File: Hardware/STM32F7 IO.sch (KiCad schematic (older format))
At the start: 19 parts, among them U16 STM32F765ZGT6

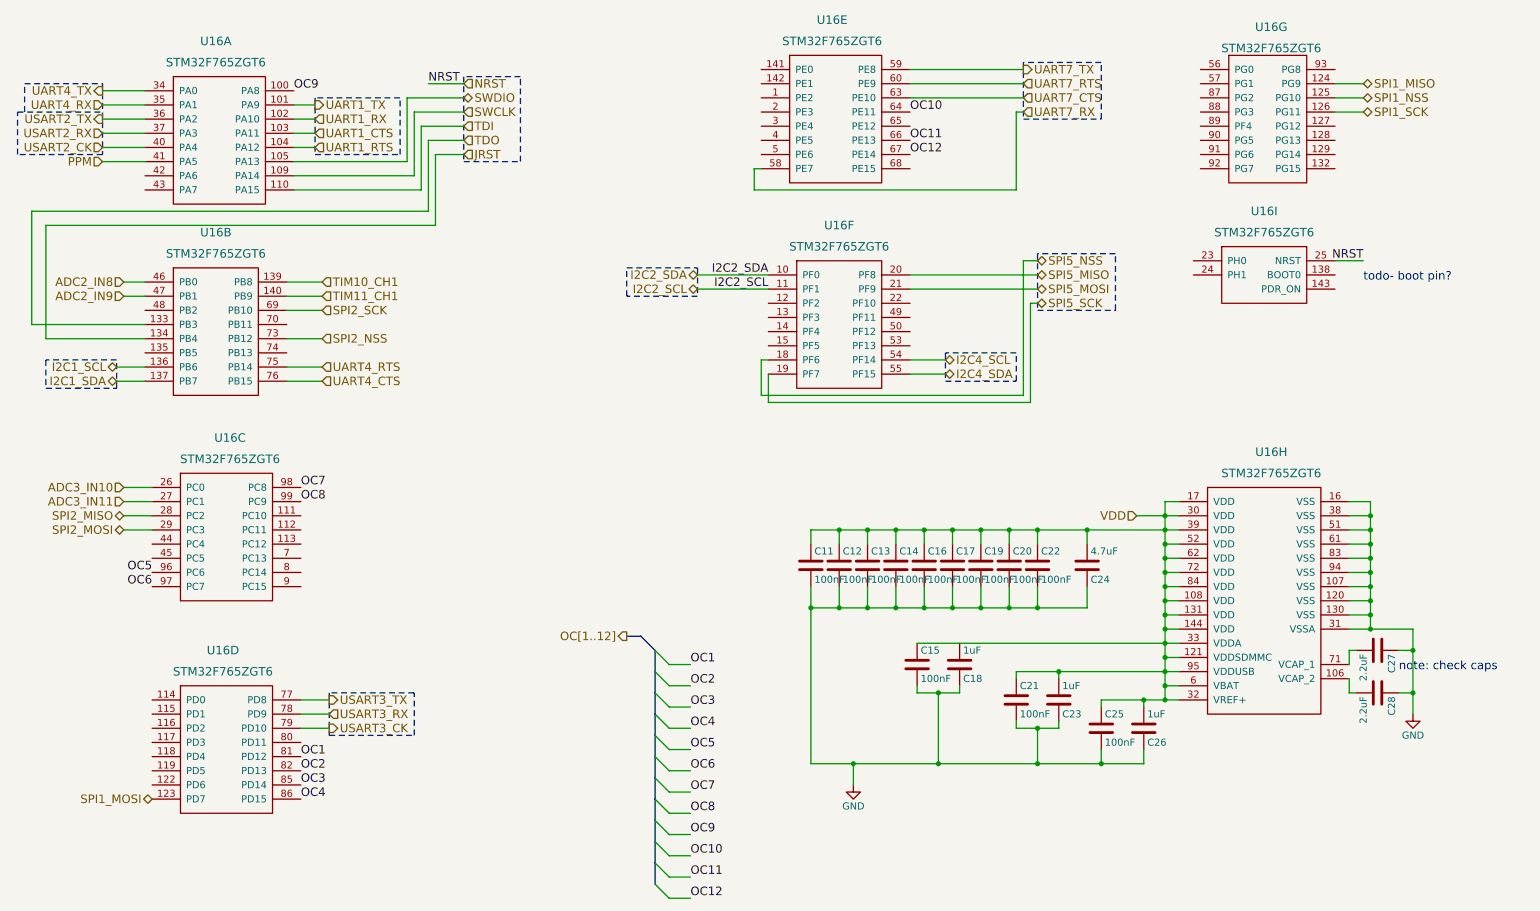
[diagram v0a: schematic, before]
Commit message: Added a lot of debug
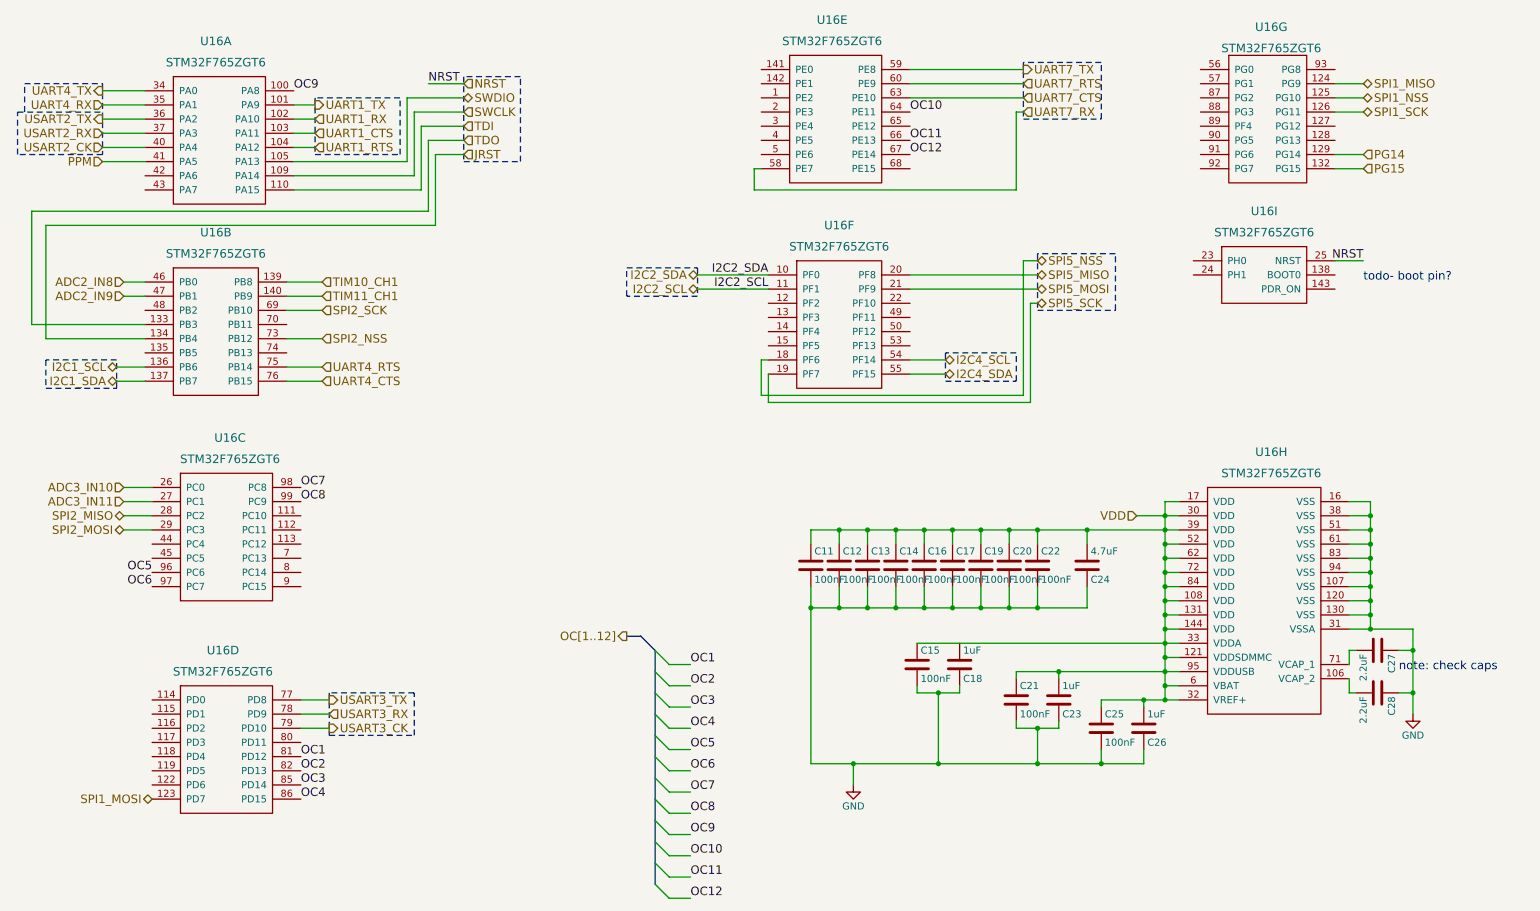
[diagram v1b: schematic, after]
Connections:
- net PG14: now reaches U16.129 (PG14)
- net PG15: now reaches U16.132 (PG15)
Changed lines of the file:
@@
 Connection ~ 7250 6350
 Wire Wire Line
-	7250 5850 7250 6350
+	7250 6350 7250 5850
 Connection ~ 7950 6100
 Connection ~ 7950 6350
 Wire Wire Line
-	7950 6100 7950 6350
+	7950 6350 7950 6100
 Connection ~ 6350 5250
 Connection ~ 8400 6350
 Wire Wire Line
-	8950 5300 8850 5300
+	8850 5300 8950 5300
 Wire Wire Line
 	7100 5850 7100 5800
 Wire Wire Line
-	7100 5850 7250 5850
-Wire Wire Line
-	7250 5850 7400 5850
+	7100 5850 7400 5850
 Wire Wire Line
 	7400 5850 7400 5800
@@
 	8700 6350 8700 6250
 Wire Wire Line
-	6350 6350 6650 6350
-Wire Wire Line
-	6650 6350 7250 6350
-Wire Wire Line
-	7250 6350 7950 6350
-Wire Wire Line
-	7950 6350 8400 6350
-Wire Wire Line
-	8400 6350 8700 6350
+	6350 6350 8700 6350
 Wire Wire Line
 	8400 6350 8400 6250
@@
 	7800 6100 7800 6050
 Wire Wire Line
-	7800 6100 7950 6100
-Wire Wire Line
-	7950 6100 8100 6100
+	7800 6100 8100 6100
 Wire Wire Line
 	8100 6100 8100 6050
 Connection ~ 8300 4700
 Wire Wire Line
-	8300 4800 8300 4700
+	8300 4700 8300 4800
 Connection ~ 7950 5250
 Wire Wire Line
@@
 Connection ~ 6750 5250
 Wire Wire Line
-	6750 5100 6750 5250
+	6750 5250 6750 5100
 Connection ~ 6950 5250
 Wire Wire Line
-	6950 5100 6950 5250
+	6950 5250 6950 5100
 Connection ~ 7150 5250
 Wire Wire Line
-	7150 5100 7150 5250
+	7150 5250 7150 5100
 Connection ~ 7350 5250
 Wire Wire Line
-	7350 5100 7350 5250
+	7350 5250 7350 5100
 Connection ~ 7550 5250
 Wire Wire Line
-	7550 5100 7550 5250
+	7550 5250 7550 5100
 Connection ~ 7750 5250
 Wire Wire Line
-	7750 5100 7750 5250
+	7750 5250 7750 5100
 Wire Wire Line
 	7950 5250 7950 5100
 Wire Wire Line
-	6350 5250 6550 5250
-Wire Wire Line
-	6550 5250 6750 5250
-Wire Wire Line
-	6750 5250 6950 5250
-Wire Wire Line
-	6950 5250 7150 5250
-Wire Wire Line
-	7150 5250 7350 5250
-Wire Wire Line
-	7350 5250 7550 5250
-Wire Wire Line
-	7550 5250 7750 5250
-Wire Wire Line
-	7750 5250 7950 5250
-Wire Wire Line
-	7950 5250 8300 5250
-Wire Wire Line
-	6350 5100 6350 5250
-Wire Wire Line
-	6350 5250 6350 6350
+	6350 5250 8300 5250
+Wire Wire Line
+	6350 5100 6350 6350
 Connection ~ 7950 4700
 Wire Wire Line
-	7950 4800 7950 4700
+	7950 4700 7950 4800
 Connection ~ 7750 4700
 Wire Wire Line
-	7750 4800 7750 4700
+	7750 4700 7750 4800
 Connection ~ 7550 4700
 Wire Wire Line
-	7550 4800 7550 4700
+	7550 4700 7550 4800
 Connection ~ 7350 4700
 Wire Wire Line
-	7350 4800 7350 4700
+	7350 4700 7350 4800
 Connection ~ 7150 4700
 Wire Wire Line
-	7150 4800 7150 4700
+	7150 4700 7150 4800
 Connection ~ 6950 4700
 Wire Wire Line
-	6950 4800 6950 4700
+	6950 4700 6950 4800
 Connection ~ 6750 4700
 Wire Wire Line
-	6750 4800 6750 4700
+	6750 4700 6750 4800
 Connection ~ 6550 4700
 Wire Wire Line
@@
 	10600 5850 10500 5850
 Wire Wire Line
-	10600 5400 10600 5550
-Wire Wire Line
-	10600 5550 10600 5850
-Wire Wire Line
-	10600 5850 10600 6000
+	10600 5400 10600 6000
 Wire Wire Line
 	10150 5550 10200 5550
@@
 Connection ~ 8850 5700
 Wire Wire Line
-	7800 5700 8100 5700
-Wire Wire Line
-	8100 5700 8850 5700
-Wire Wire Line
-	8850 5700 8950 5700
+	7800 5700 8950 5700
 Connection ~ 8850 5800
 Wire Wire Line
-	8400 5900 8700 5900
-Wire Wire Line
-	8700 5900 8850 5900
-Wire Wire Line
-	8850 5900 8950 5900
+	8400 5900 8950 5900
 Connection ~ 8850 5600
 Wire Wire Line
@@
 Connection ~ 8850 4600
 Wire Wire Line
-	8650 4600 8850 4600
-Wire Wire Line
-	8850 4600 8950 4600
+	8650 4600 8950 4600
 Connection ~ 8850 4700
 Connection ~ 8850 4800
 Wire Wire Line
-	8950 4800 8850 4800
+	8850 4800 8950 4800
 Connection ~ 8850 4900
 Wire Wire Line
-	8950 4900 8850 4900
+	8850 4900 8950 4900
 Connection ~ 8850 5000
 Wire Wire Line
-	8950 5000 8850 5000
+	8850 5000 8950 5000
 Connection ~ 8850 5100
 Wire Wire Line
-	8950 5100 8850 5100
+	8850 5100 8950 5100
 Connection ~ 8850 5200
 Wire Wire Line
-	8950 5200 8850 5200
+	8850 5200 8950 5200
 Connection ~ 8850 5300
 Wire Wire Line
-	6350 4700 6550 4700
-Wire Wire Line
-	6550 4700 6750 4700
-Wire Wire Line
-	6750 4700 6950 4700
-Wire Wire Line
-	6950 4700 7150 4700
-Wire Wire Line
-	7150 4700 7350 4700
-Wire Wire Line
-	7350 4700 7550 4700
-Wire Wire Line
-	7550 4700 7750 4700
-Wire Wire Line
-	7750 4700 7950 4700
-Wire Wire Line
-	7950 4700 8300 4700
-Wire Wire Line
-	8300 4700 8850 4700
-Wire Wire Line
-	8850 4700 8950 4700
+	6350 4700 8950 4700
 Connection ~ 8850 5400
 Wire Wire Line
-	8950 5400 8850 5400
-Wire Wire Line
-	7100 5500 8850 5500
-Wire Wire Line
-	8850 5500 8950 5500
-Wire Wire Line
-	8850 4500 8850 4600
-Wire Wire Line
-	8850 4600 8850 4700
-Wire Wire Line
-	8850 4700 8850 4800
-Wire Wire Line
-	8850 4800 8850 4900
-Wire Wire Line
-	8850 4900 8850 5000
-Wire Wire Line
-	8850 5000 8850 5100
-Wire Wire Line
-	8850 5100 8850 5200
-Wire Wire Line
-	8850 5200 8850 5300
-Wire Wire Line
-	8850 5300 8850 5400
-Wire Wire Line
-	8850 5400 8850 5500
-Wire Wire Line
-	8850 5500 8850 5600
-Wire Wire Line
-	8850 5600 8850 5700
-Wire Wire Line
-	8850 5700 8850 5800
-Wire Wire Line
-	8850 5800 8850 5900
+	8850 5400 8950 5400
+Wire Wire Line
+	7100 5500 8950 5500
+Wire Wire Line
+	8850 4500 8850 5900
 Wire Wire Line
 	8950 4500 8850 4500
@@
 Connection ~ 10300 4700
 Wire Wire Line
-	10150 4700 10300 4700
+	10300 4700 10150 4700
 Connection ~ 10300 4800
 Wire Wire Line
-	10150 4800 10300 4800
+	10300 4800 10150 4800
 Connection ~ 10300 4900
 Wire Wire Line
-	10150 4900 10300 4900
+	10300 4900 10150 4900
 Connection ~ 10300 5000
 Wire Wire Line
-	10150 5000 10300 5000
+	10300 5000 10150 5000
 Connection ~ 10300 5100
 Wire Wire Line
-	10150 5100 10300 5100
+	10300 5100 10150 5100
 Connection ~ 10300 5200
 Wire Wire Line
-	10150 5200 10300 5200
+	10300 5200 10150 5200
 Connection ~ 10300 5300
 Wire Wire Line
-	10150 5300 10300 5300
-Wire Wire Line
-	10150 5400 10300 5400
-Wire Wire Line
-	10300 5400 10600 5400
-Wire Wire Line
-	10300 4500 10300 4600
-Wire Wire Line
-	10300 4600 10300 4700
-Wire Wire Line
-	10300 4700 10300 4800
-Wire Wire Line
-	10300 4800 10300 4900
-Wire Wire Line
-	10300 4900 10300 5000
-Wire Wire Line
-	10300 5000 10300 5100
-Wire Wire Line
-	10300 5100 10300 5200
-Wire Wire Line
-	10300 5200 10300 5300
-Wire Wire Line
-	10300 5300 10300 5400
+	10300 5300 10150 5300
+Wire Wire Line
+	10150 5400 10600 5400
+Wire Wire Line
+	10300 4500 10300 5400
 Wire Wire Line
 	10150 4500 10300 4500
@@
 	5500 5650 5350 5650
 Wire Bus Line
-	5250 5550 5250 5700
-Wire Bus Line
-	5250 5700 5250 5850
-Wire Bus Line
-	5250 5850 5250 6000
-Wire Bus Line
-	5250 6000 5250 6150
-Wire Bus Line
-	5250 6150 5250 6300
-Wire Bus Line
-	5250 6300 5250 6450
-Wire Bus Line
-	5250 6450 5250 6600
-Wire Bus Line
-	5250 6600 5250 6750
-Wire Bus Line
-	5250 6750 5250 6900
-Wire Bus Line
-	5250 6900 5250 7050
-Wire Bus Line
-	5250 7050 5250 7200
+	5250 5550 5250 7200
 Wire Bus Line
 	5150 5450 5250 5550
 Wire Bus Line
 	5050 5450 5150 5450
+Text HLabel 10250 2050 2    60   Input ~ 0
+PG14
+Text HLabel 10250 2150 2    60   Input ~ 0
+PG15
+Wire Wire Line
+	10250 2050 10050 2050
+Wire Wire Line
+	10050 2150 10250 2150
 $EndSCHEMATC
